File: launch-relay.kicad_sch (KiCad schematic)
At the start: 28 parts, among them J4 Conn_01x07_Socket, U1 STM32U083KCUx, U2 MX25R3235FM1IL0, U3 BMA580

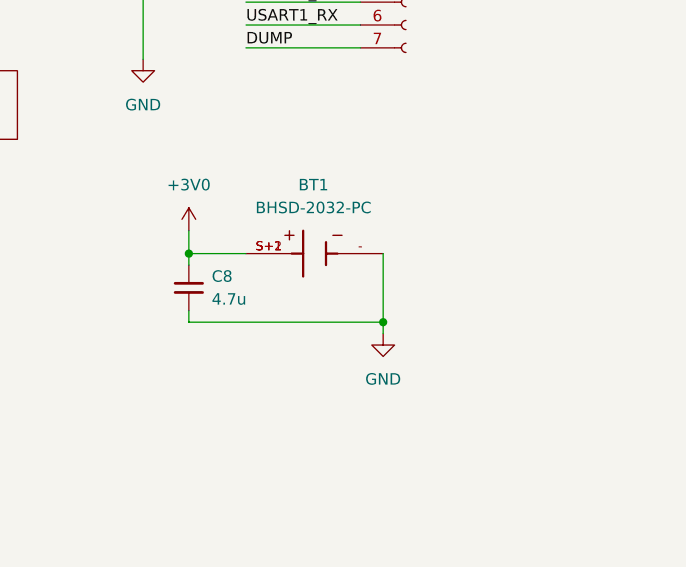
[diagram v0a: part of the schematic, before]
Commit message: fixed switch circuit
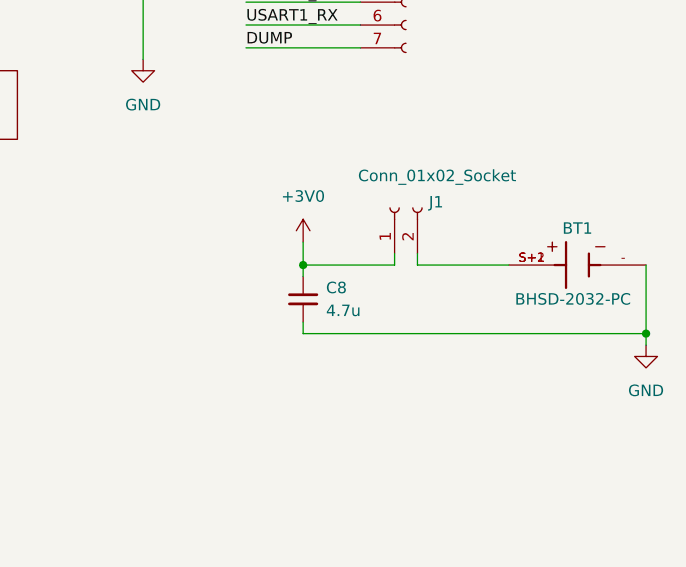
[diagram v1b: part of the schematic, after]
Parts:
- added J1: Conn_01x02_Socket, Connector_PinSocket_2.54mm:PinSocket_1x02_P2.54mm_Vertical, symbol Connector:Conn_01x02_Socket
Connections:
- net +3V0: now also J1.1 (Pin_1); no longer BT1.S+1, BT1.S+2
- new net: BT1.S+1, BT1.S+2, J1.2 (Pin_2)
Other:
- moved on the sheet: BT1, C8
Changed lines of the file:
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@@
 	(paper "A4")
 	(junction
+		(at 167.64 59.69)
+		(diameter 0)
+		(color 0 0 0 0)
+	)
+	(junction
 		(at 85.09 135.89)
 		(diameter 0)
@@
 	)
 	(junction
-		(at 176.53 66.04)
+		(at 205.74 67.31)
 		(diameter 0)
 		(color 0 0 0 0)
@@
 	)
 	(junction
-		(at 154.94 58.42)
-		(diameter 0)
-		(color 0 0 0 0)
-	)
-	(junction
 		(at 149.86 27.94)
 		(diameter 0)
@@
 	(wire
 		(pts
-			(xy 66.04 128.27) (xy 66.04 130.81)
+			(xy 177.8 59.69) (xy 167.64 59.69)
 		)
 		(stroke
@@
 	(wire
 		(pts
-			(xy 96.52 64.77) (xy 96.52 59.69)
+			(xy 66.04 128.27) (xy 66.04 130.81)
 		)
 		(stroke
@@
 	(wire
 		(pts
-			(xy 83.82 57.15) (xy 71.12 57.15)
+			(xy 96.52 64.77) (xy 96.52 59.69)
 		)
 		(stroke
@@
 	(wire
 		(pts
-			(xy 71.12 64.77) (xy 96.52 64.77)
+			(xy 83.82 57.15) (xy 71.12 57.15)
 		)
 		(stroke
@@
 	(wire
 		(pts
-			(xy 26.67 25.4) (xy 26.67 26.67)
+			(xy 71.12 64.77) (xy 96.52 64.77)
 		)
 		(stroke
@@
 	(wire
 		(pts
-			(xy 154.94 55.88) (xy 154.94 58.42)
+			(xy 26.67 25.4) (xy 26.67 26.67)
 		)
 		(stroke
@@
 	(wire
 		(pts
-			(xy 92.71 48.26) (xy 87.63 48.26)
+			(xy 180.34 59.69) (xy 190.5 59.69)
 		)
 		(stroke
@@
 	(wire
 		(pts
-			(xy 154.94 58.42) (xy 161.29 58.42)
+			(xy 92.71 48.26) (xy 87.63 48.26)
 		)
 		(stroke
@@
 	(wire
 		(pts
-			(xy 154.94 64.77) (xy 154.94 66.04)
+			(xy 167.64 66.04) (xy 167.64 67.31)
 		)
 		(stroke
@@
 	(wire
 		(pts
-			(xy 176.53 66.04) (xy 176.53 58.42)
+			(xy 205.74 67.31) (xy 205.74 59.69)
 		)
 		(stroke
@@
 	(wire
 		(pts
-			(xy 154.94 59.69) (xy 154.94 58.42)
+			(xy 167.64 57.15) (xy 167.64 59.69)
 		)
 		(stroke
@@
 	(wire
 		(pts
-			(xy 176.53 67.31) (xy 176.53 66.04)
+			(xy 205.74 68.58) (xy 205.74 67.31)
 		)
 		(stroke
@@
 	(wire
 		(pts
+			(xy 177.8 58.42) (xy 177.8 59.69)
+		)
+		(stroke
+			(width 0)
+			(type default)
+		)
+	)
+	(wire
+		(pts
 			(xy 66.04 19.05) (xy 60.96 19.05)
 		)
@@
 	(wire
 		(pts
-			(xy 154.94 66.04) (xy 176.53 66.04)
+			(xy 167.64 67.31) (xy 205.74 67.31)
 		)
 		(stroke
@@
 	(wire
 		(pts
+			(xy 167.64 59.69) (xy 167.64 60.96)
+		)
+		(stroke
+			(width 0)
+			(type default)
+		)
+	)
+	(wire
+		(pts
 			(xy 41.91 62.23) (xy 45.72 62.23)
 		)
@@
 	(wire
 		(pts
+			(xy 180.34 58.42) (xy 180.34 59.69)
+		)
+		(stroke
+			(width 0)
+			(type default)
+		)
+	)
+	(wire
+		(pts
 			(xy 120.65 130.81) (xy 120.65 134.62)
 		)
@@
 	(symbol
 		(lib_id "power:+3V0")
-		(at 154.94 55.88 0)
+		(at 167.64 57.15 0)
 		(unit 1)
 		(body_style 1)
@@
 		(fields_autoplaced yes)
 		(property "Reference" "#PWR05"
-			(at 154.94 59.69 0)
+			(at 167.64 60.96 0)
 			(hide yes)
 			(show_name no)
@@
 		)
 		(property "Value" "+3V0"
-			(at 154.94 50.8 0)
+			(at 167.64 52.07 0)
 			(show_name no)
 			(do_not_autoplace no)
@@
 		)
 		(property "Footprint" ""
-			(at 154.94 55.88 0)
+			(at 167.64 57.15 0)
 			(hide yes)
 			(show_name no)
@@
 		)
 		(property "Datasheet" ""
-			(at 154.94 55.88 0)
+			(at 167.64 57.15 0)
 			(hide yes)
 			(show_name no)
@@
 		)
 		(property "Description" "Power symbol creates a global label with name \"+3V0\""
-			(at 154.94 55.88 0)
+			(at 167.64 57.15 0)
 			(hide yes)
 			(show_name no)
@@
 	)
 	(symbol
+		(lib_id "Connector:Conn_01x02_Socket")
+		(at 177.8 53.34 90)
+		(unit 1)
+		(body_style 1)
+		(exclude_from_sim no)
+		(in_bom yes)
+		(on_board yes)
+		(in_pos_files yes)
+		(dnp no)
+		(property "Reference" "J1"
+			(at 181.61 52.7049 90)
+			(show_name no)
+			(do_not_autoplace no)
+			(effects
+				(font
+					(size 1.27 1.27)
+				)
+				(justify right)
+			)
+		)
+		(property "Value" "Conn_01x02_Socket"
+			(at 173.736 49.784 90)
+			(show_name no)
+			(do_not_autoplace no)
+			(effects
+				(font
+					(size 1.27 1.27)
+				)
+				(justify right)
+			)
+		)
+		(property "Footprint" "Connector_PinSocket_2.54mm:PinSocket_1x02_P2.54mm_Vertical"
+			(at 177.8 53.34 0)
+			(hide yes)
+			(show_name no)
+			(do_not_autoplace no)
+			(effects
+				(font
+					(size 1.27 1.27)
+				)
+			)
+		)
+		(property "Datasheet" ""
+			(at 177.8 53.34 0)
+			(hide yes)
+			(show_name no)
+			(do_not_autoplace no)
+			(effects
+				(font
+					(size 1.27 1.27)
+				)
+			)
+		)
+		(property "Description" "Generic connector, single row, 01x02, script generated"
+			(at 177.8 53.34 0)
+			(hide yes)
+			(show_name no)
+			(do_not_autoplace no)
+			(effects
+				(font
+					(size 1.27 1.27)
+				)
+			)
+		)
+		(pin "2"
+		)
+		(pin "1"
+		)
+		(instances
+			(project "launch-relay"
+				(path "/5fd10500-b703-4d79-824f-0c6e126f5ac0"
+					(reference "J1")
+					(unit 1)
+				)
+			)
+		)
+	)
+	(symbol
 		(lib_id "power:+3V0")
 		(at 15.24 55.88 0)
@@
 	(symbol
 		(lib_id "BHSD-2032-PC:BHSD-2032-PC")
-		(at 168.91 58.42 0)
+		(at 198.12 59.69 0)
 		(unit 1)
 		(body_style 1)
@@
 		(in_pos_files yes)
 		(dnp no)
-		(fields_autoplaced yes)
 		(property "Reference" "BT1"
-			(at 168.783 50.8 0)
+			(at 198.12 55.626 0)
 			(show_name no)
 			(do_not_autoplace no)
@@
 		)
 		(property "Value" "BHSD-2032-PC"
-			(at 168.783 53.34 0)
+			(at 197.612 63.5 0)
 			(show_name no)
 			(do_not_autoplace no)
@@
 		)
 		(property "Footprint" "HPRC_Connectors:BAT_BHSD-2032-PC"
-			(at 168.91 58.42 0)
+			(at 198.12 59.69 0)
 			(hide yes)
 			(show_name no)
@@
 		)
 		(property "Datasheet" ""
-			(at 168.91 58.42 0)
+			(at 198.12 59.69 0)
 			(hide yes)
 			(show_name no)
@@
 		)
 		(property "Description" ""
-			(at 168.91 58.42 0)
+			(at 198.12 59.69 0)
 			(hide yes)
 			(show_name no)
@@
 		)
 		(property "PARTREV" "K"
-			(at 168.91 58.42 0)
+			(at 198.12 59.69 0)
 			(hide yes)
 			(show_name no)
@@
 		)
 		(property "STANDARD" "Manufacturer Recommendations"
-			(at 168.91 58.42 0)
+			(at 198.12 59.69 0)
 			(hide yes)
 			(show_name no)
@@
 		)
 		(property "MAXIMUM_PACKAGE_HEIGHT" "4.75 mm"
-			(at 168.91 58.42 0)
+			(at 198.12 59.69 0)
 			(hide yes)
 			(show_name no)
@@
 		)
 		(property "MANUFACTURER" "MPD"
-			(at 168.91 58.42 0)
+			(at 198.12 59.69 0)
 			(hide yes)
 			(show_name no)
@@
 	(symbol
 		(lib_id "Device:C_Small")
-		(at 154.94 62.23 180)
+		(at 167.64 63.5 180)
 		(unit 1)
 		(body_style 1)
@@
 		(fields_autoplaced yes)
 		(property "Reference" "C8"
-			(at 157.48 60.9599 0)
+			(at 170.18 62.2299 0)
 			(show_name no)
 			(do_not_autoplace no)
@@
 		)
 		(property "Value" "4.7u"
-			(at 157.48 63.4999 0)
+			(at 170.18 64.7699 0)
 			(show_name no)
 			(do_not_autoplace no)
@@
 		)
 		(property "Footprint" "Capacitor_SMD:C_0603_1608Metric"
-			(at 154.94 62.23 0)
+			(at 167.64 63.5 0)
 			(hide yes)
 			(show_name no)
@@
 		)
 		(property "Datasheet" ""
-			(at 154.94 62.23 0)
+			(at 167.64 63.5 0)
 			(hide yes)
 			(show_name no)
@@
 		)
 		(property "Description" "Unpolarized capacitor, small symbol"
-			(at 154.94 52.07 0)
+			(at 167.64 53.34 0)
 			(hide yes)
 			(show_name no)
@@
 	(symbol
 		(lib_id "power:GND")
-		(at 176.53 67.31 0)
+		(at 205.74 68.58 0)
 		(unit 1)
 		(body_style 1)
@@
 		(fields_autoplaced yes)
 		(property "Reference" "#PWR01"
-			(at 176.53 73.66 0)
+			(at 205.74 74.93 0)
 			(hide yes)
 			(show_name no)
@@
 		)
 		(property "Value" "GND"
-			(at 176.53 72.39 0)
+			(at 205.74 73.66 0)
 			(show_name no)
 			(do_not_autoplace no)
@@
 		)
 		(property "Footprint" ""
-			(at 176.53 67.31 0)
+			(at 205.74 68.58 0)
 			(hide yes)
 			(show_name no)
@@
 		)
 		(property "Datasheet" ""
-			(at 176.53 67.31 0)
+			(at 205.74 68.58 0)
 			(hide yes)
 			(show_name no)
@@
 		)
 		(property "Description" "Power symbol creates a global label with name \"GND\" , ground"
-			(at 176.53 67.31 0)
+			(at 205.74 68.58 0)
 			(hide yes)
 			(show_name no)
